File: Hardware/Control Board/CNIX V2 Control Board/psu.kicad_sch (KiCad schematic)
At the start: 39 parts, among them J100 HT_en, Q100 MMBTA42, Q101 IRF7820, U100 UCC3803

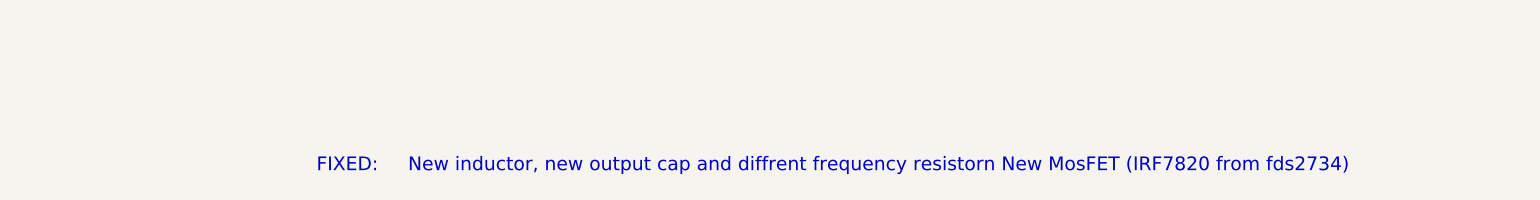
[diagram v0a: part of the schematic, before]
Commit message: cleanup of project data and files
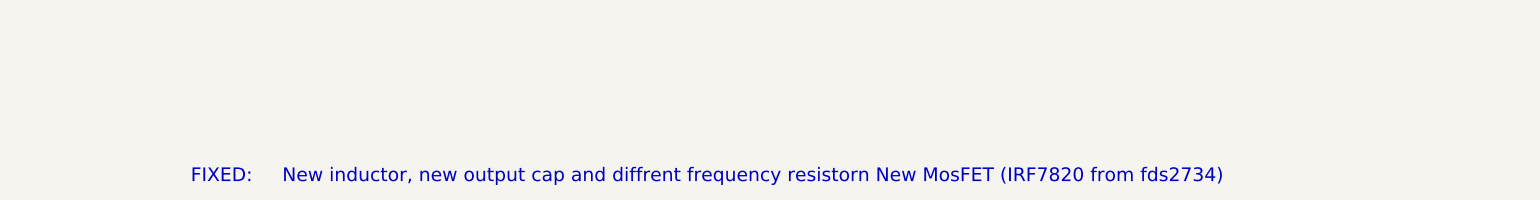
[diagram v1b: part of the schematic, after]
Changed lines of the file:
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@@
 	(title_block
 		(title "High voltage Tube PSU")
-		(date "2024-10-17")
-		(rev "2.0")
+		(date "2026-10-01")
+		(rev "2.3.0")
 		(company "C-Audio")
 	)
 	(text "FIXED: 	New inductor, new output cap and diffrent frequency resistorn New MosFET (IRF7820 from fds2734)\n"
 		(exclude_from_sim no)
-		(at 167.894 160.02 0)
+		(at 144.526 162.052 0)
 		(effects
 			(font
